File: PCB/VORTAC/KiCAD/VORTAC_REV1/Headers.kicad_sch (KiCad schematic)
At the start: 9 parts, among them J1 DEBUG, J14 918-418K2023S40001, J15 STEPPER, J3 Conn_02x02_Odd_Even

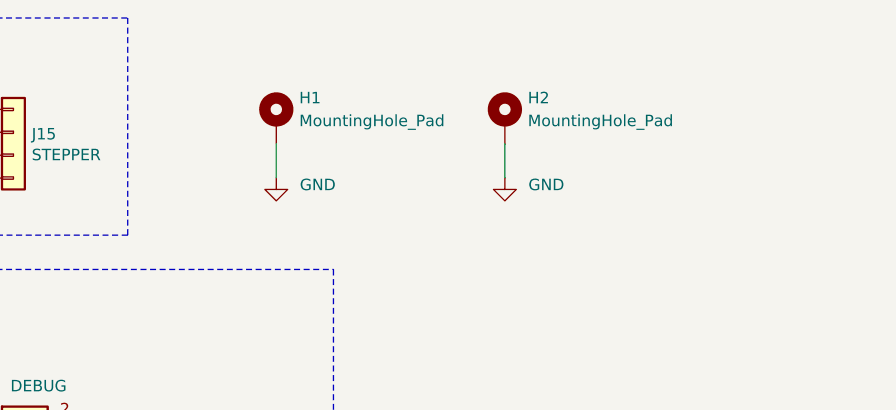
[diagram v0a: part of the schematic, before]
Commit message: FML
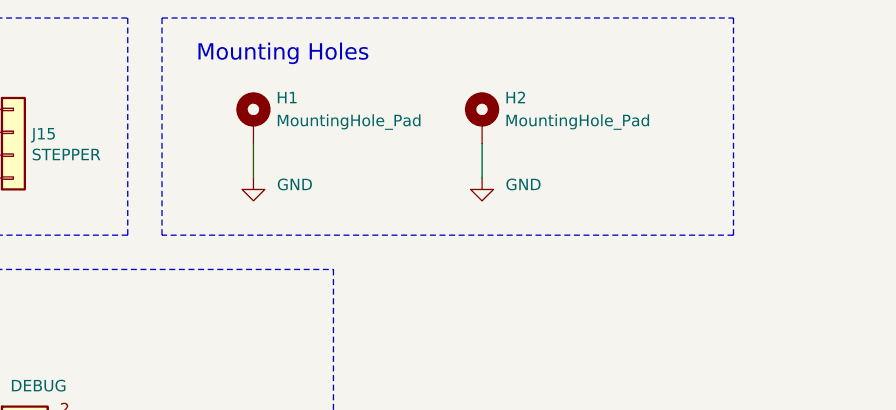
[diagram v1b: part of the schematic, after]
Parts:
- H1, H2: footprint Vortac:MountingHole_2.2mm_M2_Pad_Via_netless -> Vortac:MountingHole_2.2mm_M2_Pad_Via_NTR
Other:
- note added: "Mounting Holes"
- moved on the sheet: H1, H2
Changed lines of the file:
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@@
+		)
+	)
+	(text "Mounting Holes\n"
+		(exclude_from_sim no)
+		(at 68.58 21.59 0)
+		(effects
+			(font
+				(size 1.8034 1.8034)
+			)
+			(justify left bottom)
 		)
 	)
@@
 	(wire
 		(pts
-			(xy 77.47 30.48) (xy 77.47 34.29)
+			(xy 74.93 30.48) (xy 74.93 34.29)
 		)
 		(stroke
@@
 	(polyline
 		(pts
+			(xy 64.77 16.51) (xy 128.27 16.51)
+		)
+		(stroke
+			(width 0)
+			(type dash)
+		)
+	)
+	(polyline
+		(pts
 			(xy 16.51 123.19) (xy 16.51 83.82)
 		)
@@
 	(wire
 		(pts
-			(xy 102.87 30.48) (xy 102.87 34.29)
+			(xy 100.33 30.48) (xy 100.33 34.29)
 		)
 		(stroke
@@
 		)
 	)
+	(polyline
+		(pts
+			(xy 128.27 40.64) (xy 64.77 40.64)
+		)
+		(stroke
+			(width 0)
+			(type dash)
+		)
+	)
 	(wire
 		(pts
@@
 		)
 	)
+	(polyline
+		(pts
+			(xy 64.77 40.64) (xy 64.77 16.51)
+		)
+		(stroke
+			(width 0)
+			(type dash)
+		)
+	)
 	(wire
 		(pts
@@
 			(width 0)
 			(type default)
+		)
+	)
+	(polyline
+		(pts
+			(xy 128.27 16.51) (xy 128.27 40.64)
+		)
+		(stroke
+			(width 0)
+			(type dash)
 		)
 	)
@@
 	(symbol
 		(lib_id "power:GND")
-		(at 102.87 34.29 0)
+		(at 100.33 34.29 0)
 		(unit 1)
 		(exclude_from_sim no)
@@
 		(dnp no)
 		(property "Reference" "#PWR29"
-			(at 102.87 40.64 0)
+			(at 100.33 40.64 0)
 			(effects
 				(font
@@
 		)
 		(property "Value" "GND"
-			(at 109.474 35.052 0)
+			(at 106.934 35.052 0)
 			(effects
 				(font
@@
 		)
 		(property "Footprint" ""
-			(at 102.87 34.29 0)
+			(at 100.33 34.29 0)
 			(effects
 				(font
@@
 		)
 		(property "Datasheet" ""
-			(at 102.87 34.29 0)
+			(at 100.33 34.29 0)
 			(effects
 				(font
@@
 		)
 		(property "Description" "Power symbol creates a global label with name \"GND\" , ground"
-			(at 102.87 34.29 0)
+			(at 100.33 34.29 0)
 			(effects
 				(font
@@
 	(symbol
 		(lib_id "Mechanical:MountingHole_Pad")
-		(at 77.47 27.94 0)
+		(at 74.93 27.94 0)
 		(unit 1)
 		(exclude_from_sim no)
@@
 		(on_board yes)
 		(dnp no)
-		(fields_autoplaced yes)
 		(property "Reference" "H1"
-			(at 80.01 25.3999 0)
+			(at 77.47 25.3999 0)
 			(effects
 				(font
@@
 		)
 		(property "Value" "MountingHole_Pad"
-			(at 80.01 27.9399 0)
+			(at 77.47 27.9399 0)
 			(effects
 				(font
@@
 			)
 		)
-		(property "Footprint" "Vortac:MountingHole_2.2mm_M2_Pad_Via_netless"
-			(at 77.47 27.94 0)
+		(property "Footprint" "Vortac:MountingHole_2.2mm_M2_Pad_Via_NTR"
+			(at 74.93 27.94 0)
 			(effects
 				(font
@@
 		)
 		(property "Datasheet" "~"
-			(at 77.47 27.94 0)
+			(at 74.93 27.94 0)
 			(effects
 				(font
@@
 		)
 		(property "Description" "Mounting Hole with connection"
-			(at 77.47 27.94 0)
+			(at 74.93 27.94 0)
 			(effects
 				(font
@@
 	(symbol
 		(lib_id "power:GND")
-		(at 77.47 34.29 0)
+		(at 74.93 34.29 0)
 		(unit 1)
 		(exclude_from_sim no)
@@
 		(dnp no)
 		(property "Reference" "#PWR27"
-			(at 77.47 40.64 0)
+			(at 74.93 40.64 0)
 			(effects
 				(font
@@
 		)
 		(property "Value" "GND"
-			(at 84.074 35.052 0)
+			(at 81.534 35.052 0)
 			(effects
 				(font
@@
 		)
 		(property "Footprint" ""
-			(at 77.47 34.29 0)
+			(at 74.93 34.29 0)
 			(effects
 				(font
@@
 		)
 		(property "Datasheet" ""
-			(at 77.47 34.29 0)
+			(at 74.93 34.29 0)
 			(effects
 				(font
@@
 		)
 		(property "Description" "Power symbol creates a global label with name \"GND\" , ground"
-			(at 77.47 34.29 0)
+			(at 74.93 34.29 0)
 			(effects
 				(font
@@
 	(symbol
 		(lib_id "Mechanical:MountingHole_Pad")
-		(at 102.87 27.94 0)
+		(at 100.33 27.94 0)
 		(unit 1)
 		(exclude_from_sim no)
@@
 		(fields_autoplaced yes)
 		(property "Reference" "H2"
-			(at 105.41 25.3999 0)
+			(at 102.87 25.3999 0)
 			(effects
 				(font
@@
 		)
 		(property "Value" "MountingHole_Pad"
-			(at 105.41 27.9399 0)
+			(at 102.87 27.9399 0)
 			(effects
 				(font
@@
 			)
 		)
-		(property "Footprint" "Vortac:MountingHole_2.2mm_M2_Pad_Via_netless"
-			(at 102.87 27.94 0)
+		(property "Footprint" "Vortac:MountingHole_2.2mm_M2_Pad_Via_NTR"
+			(at 100.33 27.94 0)
 			(effects
 				(font
@@
 		)
 		(property "Datasheet" "~"
-			(at 102.87 27.94 0)
+			(at 100.33 27.94 0)
 			(effects
 				(font
@@
 		)
 		(property "Description" "Mounting Hole with connection"
-			(at 102.87 27.94 0)
-			(effects
-				(font
+			(at 100.33 27.94 0)
+			(effects
+				(font

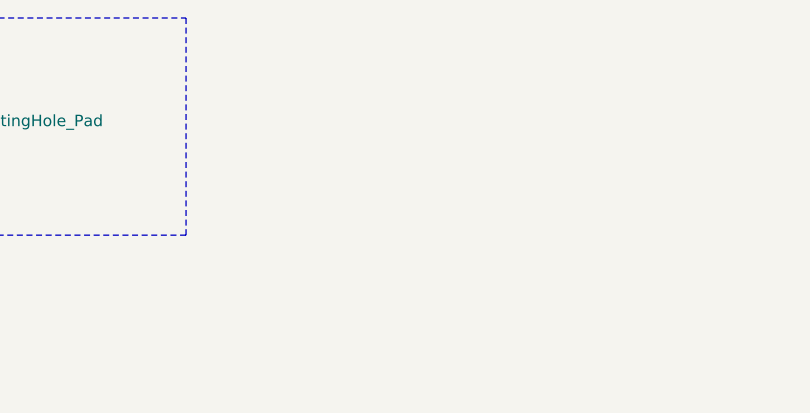
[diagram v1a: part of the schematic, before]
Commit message: USB C Pain
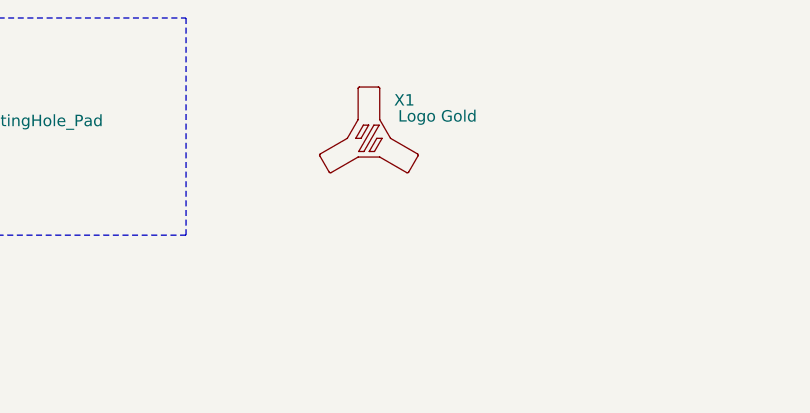
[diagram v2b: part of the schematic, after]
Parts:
- added X1: Logo Gold, Vortac:VORTAC_Logo_Gold, symbol Vortac:VORTAC_Logo
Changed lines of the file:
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@@
+	)
+	(symbol
+		(lib_id "Vortac:VORTAC_Logo")
+		(at 148.59 29.21 0)
+		(unit 1)
+		(exclude_from_sim no)
+		(in_bom yes)
+		(on_board yes)
+		(dnp no)
+		(property "Reference" "X1"
+			(at 151.384 25.654 0)
+			(effects
+				(font
+					(size 1.27 1.27)
+				)
+				(justify left)
+			)
+		)
+		(property "Value" "Logo Gold"
+			(at 156.21 27.432 0)
+			(effects
+				(font
+					(size 1.27 1.27)
+				)
+			)
+		)
+		(property "Footprint" "Vortac:VORTAC_Logo_Gold"
+			(at 148.59 29.21 0)
+			(effects
+				(font
+					(size 1.27 1.27)
+				)
+				(hide yes)
+			)
+		)
+		(property "Datasheet" ""
+			(at 148.59 29.21 0)
+			(effects
+				(font
+					(size 1.27 1.27)
+				)
+				(hide yes)
+			)
+		)
+		(property "Description" ""
+			(at 148.59 29.21 0)
+			(effects
+				(font
+					(size 1.27 1.27)
+				)
+				(hide yes)
+			)
+		)
+		(instances
+			(project ""
+				(path "/ed58d858-d9f9-4504-a982-ccfc7f9efbad/00000000-0000-0000-0000-0000613db78d"
+					(reference "X1")
+					(unit 1)
+				)
+			)
+		)
 	)
 	(symbol

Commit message: idk
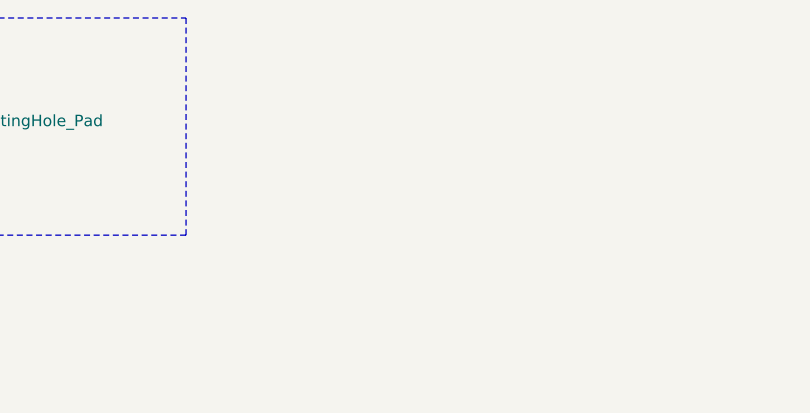
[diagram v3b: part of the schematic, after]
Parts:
- removed X1: Logo Gold, Vortac:VORTAC_Logo_Gold, symbol Vortac:VORTAC_Logo
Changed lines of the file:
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@@
-	)
-	(symbol
-		(lib_id "Vortac:VORTAC_Logo")
-		(at 148.59 29.21 0)
-		(unit 1)
-		(exclude_from_sim no)
-		(in_bom yes)
-		(on_board yes)
-		(dnp no)
-		(property "Reference" "X1"
-			(at 151.384 25.654 0)
-			(effects
-				(font
-					(size 1.27 1.27)
-				)
-				(justify left)
-			)
-		)
-		(property "Value" "Logo Gold"
-			(at 156.21 27.432 0)
-			(effects
-				(font
-					(size 1.27 1.27)
-				)
-			)
-		)
-		(property "Footprint" "Vortac:VORTAC_Logo_Gold"
-			(at 148.59 29.21 0)
-			(effects
-				(font
-					(size 1.27 1.27)
-				)
-				(hide yes)
-			)
-		)
-		(property "Datasheet" ""
-			(at 148.59 29.21 0)
-			(effects
-				(font
-					(size 1.27 1.27)
-				)
-				(hide yes)
-			)
-		)
-		(property "Description" ""
-			(at 148.59 29.21 0)
-			(effects
-				(font
-					(size 1.27 1.27)
-				)
-				(hide yes)
-			)
-		)
-		(instances
-			(project ""
-				(path "/ed58d858-d9f9-4504-a982-ccfc7f9efbad/00000000-0000-0000-0000-0000613db78d"
-					(reference "X1")
-					(unit 1)
-				)
-			)
-		)
 	)
 	(symbol
